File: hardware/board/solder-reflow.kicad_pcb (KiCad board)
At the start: 2 copper layers, 128.3 x 63.5 mm, 55 parts, among them J1 AC_Con, J2 OLED 0.91, J3 PTC_Con, J4 Barrel_Jack_Switch_Pin3Ring, K1 G3MB202PDC12, Q1 BC557, SW1 RotaryEncoder_Switch, U1 TL431LP, U2 OPA2134, U3 OPA2134, U4 L7805, U5 WeMos_D1_mini

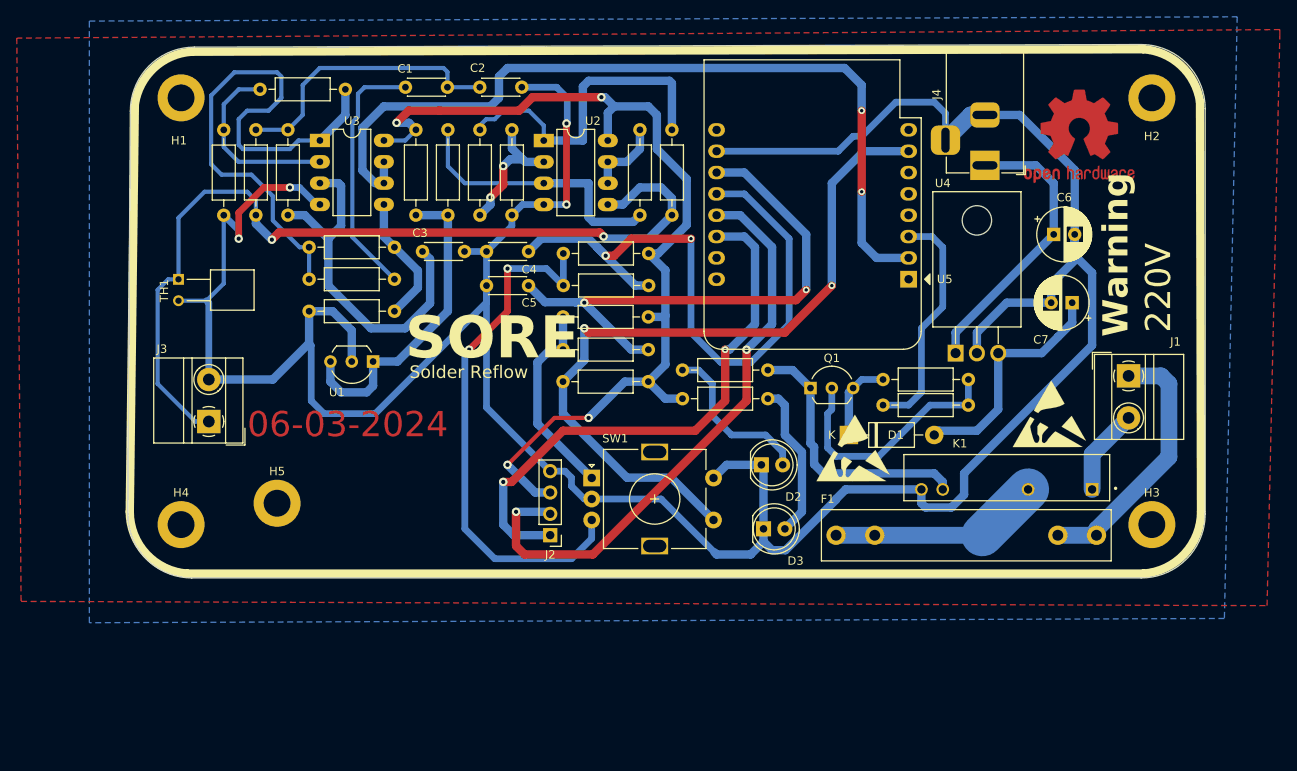
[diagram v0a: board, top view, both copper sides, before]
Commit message: [6-7-1245] finish first layout, need to review
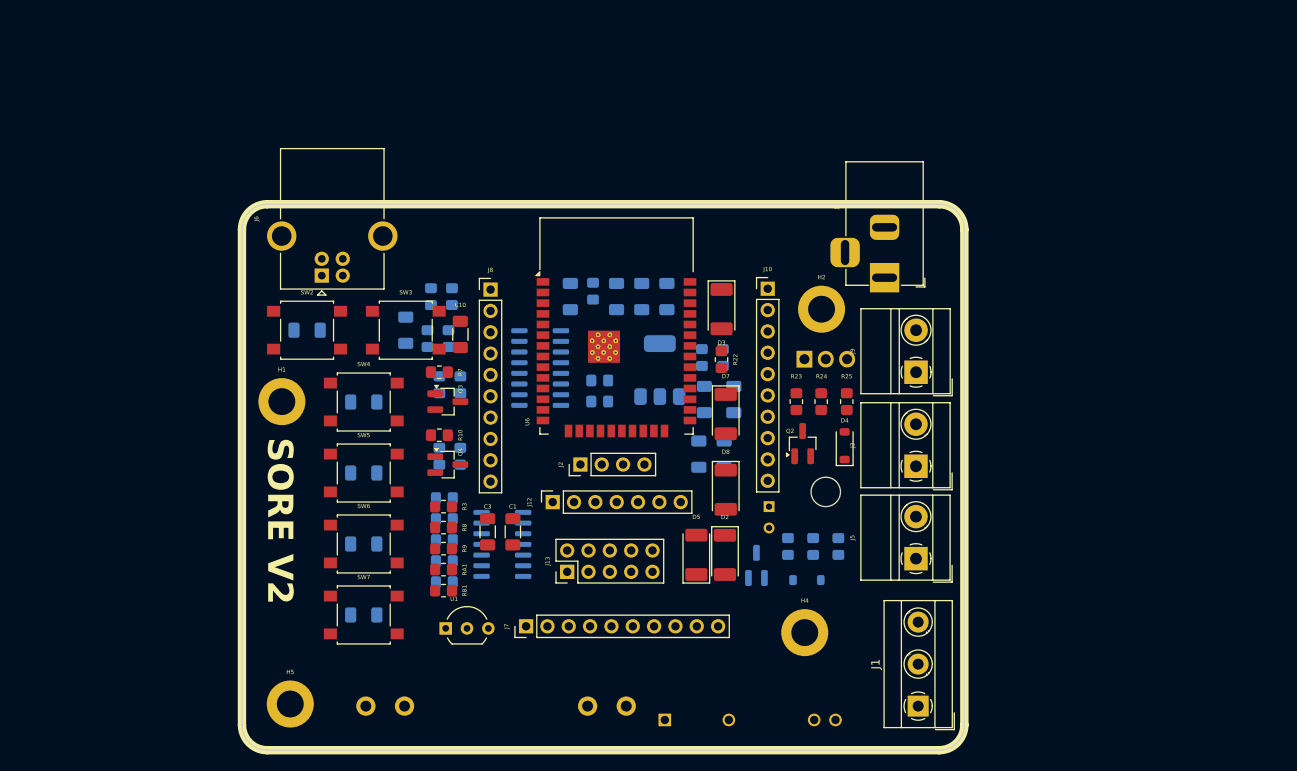
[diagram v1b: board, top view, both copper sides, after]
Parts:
- removed C4, C5: 10nF, Capacitor_THT:C_Disc_D4.3mm_W1.9mm_P5.00mm
- removed H3: MountingHole_Pad, MountingHole:MountingHole_3.2mm_M3_DIN965_Pad
- removed R11, R21: 10k, Resistor_THT:R_Axial_DIN0207_L6.3mm_D2.5mm_P10.16mm_Horizontal
- removed REF**: OSHW-Logo2_14.6x12mm_Copper, Symbol:OSHW-Logo2_14.6x12mm_Copper
- removed REF** (x2): ESD-Logo_8.9x8mm_SilkScreen, Symbol:ESD-Logo_8.9x8mm_SilkScreen
- removed REF**: Gauge_10mm_Type5_SilkScreenTop, Calibration_Scale:Gauge_10mm_Type5_SilkScreenTop
- removed SW1: RotaryEncoder_Switch, Rotary_Encoder:RotaryEncoder_Alps_EC11E-Switch_Vertical_H20mm
- removed U5: WeMos_D1_mini, Module:WEMOS_D1_mini_light
- added C10: 100nF, Capacitor_SMD:C_1206_3216Metric_Pad1.33x1.80mm_HandSolder, F.Cu at (128.5, 81.5)
- added C11: 100nF, Capacitor_SMD:C_1206_3216Metric_Pad1.33x1.80mm_HandSolder, B.Cu at (141.6, 77.0)
- added C12: 100nF, Capacitor_SMD:C_1206_3216Metric_Pad1.33x1.80mm_HandSolder, B.Cu at (150.1, 77.0)
- added C13: 22uF, Capacitor_SMD:C_1206_3216Metric_Pad1.33x1.80mm_HandSolder, B.Cu at (147.1, 77.0)
- added C14: 100nF, Capacitor_SMD:C_1206_3216Metric_Pad1.33x1.80mm_HandSolder, B.Cu at (110.2, 81.0)
- added C15: 100nF, Capacitor_SMD:C_1206_3216Metric_Pad1.33x1.80mm_HandSolder, B.Cu at (122.0, 81.0)
- added C16: 1uF, Capacitor_SMD:C_1206_3216Metric_Pad1.33x1.80mm_HandSolder, B.Cu at (117.0, 89.5)
- added C17: 1uF, Capacitor_SMD:C_1206_3216Metric_Pad1.33x1.80mm_HandSolder, B.Cu at (117.0, 98.0)
- added C18: 1uF, Capacitor_SMD:C_1206_3216Metric_Pad1.33x1.80mm_HandSolder, B.Cu at (117.0, 106.5)
- added C19: 1uF, Capacitor_SMD:C_1206_3216Metric_Pad1.33x1.80mm_HandSolder, B.Cu at (117.0, 114.9)
- added C8: 22uF, Capacitor_SMD:C_1206_3216Metric_Pad1.33x1.80mm_HandSolder, B.Cu at (159.9, 95.8)
- added C9: 22uF, Capacitor_SMD:C_1206_3216Metric_Pad1.33x1.80mm_HandSolder, B.Cu at (156.9, 95.8)
- added D4: 1N4001, Diode_SMD:D_SOD-123, F.Cu at (174.2, 94.8)
- added D5: SSR2, LED_SMD:LED_2010_5025Metric_Pad1.52x2.65mm_HandSolder, F.Cu at (156.6, 107.7)
- added D7: TXD, LED_SMD:LED_2010_5025Metric_Pad1.52x2.65mm_HandSolder, F.Cu at (160.1, 91.0)
- added D8: RXD, LED_SMD:LED_2010_5025Metric_Pad1.52x2.65mm_HandSolder, F.Cu at (160.1, 100.0)
- added J10: PINOUT, Connector_PinHeader_2.54mm:PinHeader_1x10_P2.54mm_Vertical, F.Cu at (165.1, 76.1)
- added J12: ST7789, Connector_PinSocket_2.54mm:PinSocket_1x07_P2.54mm_Vertical, F.Cu at (139.5, 101.5)
- added J13: JTAG10, Connector_PinHeader_2.54mm:PinHeader_2x05_P2.54mm_Vertical, F.Cu at (141.2, 109.8)
- added J5: SSROUT2, TerminalBlock_MetzConnect:TerminalBlock_MetzConnect_Type011_RT05502HBWC_1x02_P5.00mm_Horizontal, F.Cu at (182.7, 108.2)
- added J6: USB_B, Connector_USB:USB_B_OST_USB-B1HSxx_Horizontal, F.Cu at (112.0, 74.5)
- added J7: PINOUT, Connector_PinHeader_2.54mm:PinHeader_1x10_P2.54mm_Vertical, F.Cu at (136.3, 116.2)
- added J8: PINOUT, Connector_PinHeader_2.54mm:PinHeader_1x10_P2.54mm_Vertical, F.Cu at (132.1, 76.2)
- added J9: 12VIN, TerminalBlock_MetzConnect:TerminalBlock_MetzConnect_Type011_RT05502HBWC_1x02_P5.00mm_Horizontal, F.Cu at (182.8, 86.0)
- added Q2: SS8550, Package_TO_SOT_SMD:SOT-23_Handsoldering, F.Cu at (169.2, 94.5)
- added Q3: SS8050, Package_TO_SOT_SMD:SOT-23_Handsoldering, F.Cu at (127.0, 89.5)
- added Q4: SS8050, Package_TO_SOT_SMD:SOT-23_Handsoldering, F.Cu at (127.0, 97.0)
- added R23: 10k, Resistor_SMD:R_0805_2012Metric_Pad1.20x1.40mm_HandSolder, F.Cu at (168.5, 89.5)
- added R24: 10k, Resistor_SMD:R_0805_2012Metric_Pad1.20x1.40mm_HandSolder, F.Cu at (171.4, 89.5)
- added R25: 1k, Resistor_SMD:R_0805_2012Metric_Pad1.20x1.40mm_HandSolder, F.Cu at (174.5, 89.5)
- added R26: 1k, Resistor_SMD:R_0805_2012Metric_Pad1.20x1.40mm_HandSolder, B.Cu at (157.2, 84.2)
- added R27: 1k, Resistor_SMD:R_0805_2012Metric_Pad1.20x1.40mm_HandSolder, B.Cu at (159.8, 84.2)
- added R28: 1k, Resistor_SMD:R_0805_2012Metric_Pad1.20x1.40mm_HandSolder, B.Cu at (144.3, 76.3)
- added R29: 22k, Resistor_SMD:R_0805_2012Metric_Pad1.20x1.40mm_HandSolder, B.Cu at (128.5, 87.5)
- added R30: 22k, Resistor_SMD:R_0805_2012Metric_Pad1.20x1.40mm_HandSolder, B.Cu at (127.1, 82.0)
- added R31: 22k, Resistor_SMD:R_0805_2012Metric_Pad1.20x1.40mm_HandSolder, B.Cu at (127.5, 77.0)
- added R32: 22k, Resistor_SMD:R_0805_2012Metric_Pad1.20x1.40mm_HandSolder, B.Cu at (128.5, 96.0)
- added RA1: 25k, Resistor_SMD:R_0805_2012Metric_Pad1.20x1.40mm_HandSolder, F.Cu at (126.5, 109.5)
- added RB1: 25k, Resistor_SMD:R_0805_2012Metric_Pad1.20x1.40mm_HandSolder, F.Cu at (126.5, 112.0)
- added SW2: RST, Button_Switch_SMD:SW_SPST_B3S-1000, F.Cu at (110.2, 81.0)
- added SW3: IO0, Button_Switch_SMD:SW_SPST_B3S-1000, F.Cu at (122.0, 81.0)
- added SW4: IO0, Button_Switch_SMD:SW_SPST_B3S-1000, F.Cu at (117.0, 89.5)
- added SW5: IO0, Button_Switch_SMD:SW_SPST_B3S-1000, F.Cu at (117.0, 98.0)
- added SW6: IO0, Button_Switch_SMD:SW_SPST_B3S-1000, F.Cu at (117.0, 106.5)
- added SW7: IO0, Button_Switch_SMD:SW_SPST_B3S-1000, F.Cu at (117.0, 114.9)
- added U6: ESP32-WROOM-32D, RF_Module:ESP32-WROOM-32D, F.Cu at (147.1, 83.5)
- added U7: CH340C, Package_SO:SOIC-16_3.9x9.9mm_P1.27mm, B.Cu at (138.0, 85.5)
- C1: value 68nF -> 1nF; footprint Capacitor_THT:C_Disc_D4.3mm_W1.9mm_P5.00mm -> Capacitor_SMD:C_1206_3216Metric_Pad1.33x1.80mm_HandSolder
- C2: value 390nF -> 1uF; footprint Capacitor_THT:C_Disc_D4.3mm_W1.9mm_P5.00mm -> Capacitor_SMD:C_1206_3216Metric_Pad1.33x1.80mm_HandSolder; moved to B.Cu
- C3: value 180nF -> 1nF; footprint Capacitor_THT:C_Disc_D4.3mm_W1.9mm_P5.00mm -> Capacitor_SMD:C_1206_3216Metric_Pad1.33x1.80mm_HandSolder
- C6, C7: footprint Capacitor_THT:CP_Radial_D6.3mm_P2.50mm -> Capacitor_SMD:C_1206_3216Metric_Pad1.33x1.80mm_HandSolder; moved to B.Cu
- D1: footprint Diode_THT:D_DO-41_SOD81_P10.16mm_Horizontal -> Diode_SMD:D_SOD-123; moved to B.Cu
- D2: value SSR -> SSR1; footprint LED_THT:LED_D5.0mm -> LED_SMD:LED_2010_5025Metric_Pad1.52x2.65mm_HandSolder
- D3: footprint LED_THT:LED_D5.0mm -> LED_SMD:LED_2010_5025Metric_Pad1.52x2.65mm_HandSolder
- F1, K1, TH1, U4: moved to B.Cu
- J1: value AC_Con -> ACCON; footprint TerminalBlock_MetzConnect:TerminalBlock_MetzConnect_Type011_RT05502HBWC_1x02_P5.00mm_Horizontal -> TerminalBlock_MetzConnect:TerminalBlock_MetzConnect_Type055_RT01503HDWU_1x03_P5.00mm_Horizontal
- J4: value Barrel_Jack_Switch_Pin3Ring -> 12V
- Q1: value BC557 -> SS8550; footprint Package_TO_SOT_THT:TO-92_Inline_Wide -> Package_TO_SOT_SMD:SOT-23_Handsoldering; moved to B.Cu
- R1, R14, R15, R16, R17, R18, R19, R2, R20, R4, R5, R6: footprint Resistor_THT:R_Axial_DIN0207_L6.3mm_D2.5mm_P10.16mm_Horizontal -> Resistor_SMD:R_0805_2012Metric_Pad1.20x1.40mm_HandSolder; moved to B.Cu
- R10: value 5.1K -> 10k; footprint Resistor_THT:R_Axial_DIN0207_L6.3mm_D2.5mm_P10.16mm_Horizontal -> Resistor_SMD:R_0805_2012Metric_Pad1.20x1.40mm_HandSolder
- R12: value 3.09k -> 4K7; footprint Resistor_THT:R_Axial_DIN0207_L6.3mm_D2.5mm_P10.16mm_Horizontal -> Resistor_SMD:R_0805_2012Metric_Pad1.20x1.40mm_HandSolder; moved to B.Cu
- R13: value 20k -> 4K7; footprint Resistor_THT:R_Axial_DIN0207_L6.3mm_D2.5mm_P10.16mm_Horizontal -> Resistor_SMD:R_0805_2012Metric_Pad1.20x1.40mm_HandSolder; moved to B.Cu
- R22, R3: footprint Resistor_THT:R_Axial_DIN0207_L6.3mm_D2.5mm_P10.16mm_Horizontal -> Resistor_SMD:R_0805_2012Metric_Pad1.20x1.40mm_HandSolder
- R7: value 1k -> 10k; footprint Resistor_THT:R_Axial_DIN0207_L6.3mm_D2.5mm_P10.16mm_Horizontal -> Resistor_SMD:R_0805_2012Metric_Pad1.20x1.40mm_HandSolder
- R8: value 17.4k -> 16k; footprint Resistor_THT:R_Axial_DIN0207_L6.3mm_D2.5mm_P10.16mm_Horizontal -> Resistor_SMD:R_0805_2012Metric_Pad1.20x1.40mm_HandSolder
- R9: value 107k -> 16k; footprint Resistor_THT:R_Axial_DIN0207_L6.3mm_D2.5mm_P10.16mm_Horizontal -> Resistor_SMD:R_0805_2012Metric_Pad1.20x1.40mm_HandSolder
- U2: value OPA2134 -> TL074; footprint Package_DIP:DIP-8_W7.62mm_LongPads -> Package_SO:SOIC-14_3.9x8.7mm_P1.27mm; moved to B.Cu
- U3: value OPA2134 -> AMS1117-3.3; footprint Package_DIP:DIP-8_W7.62mm_LongPads -> Package_TO_SOT_SMD:SOT-223-3_TabPin2; moved to B.Cu
- moved J3 84.4 mm to (182.7, 97.2)
- moved H4 75.4 mm to (169.5, 117.0)
- moved TH1 75.3 mm to (165.2, 102.0)
- moved R1 54.0 mm to (126.6, 111.0), turned to 180 degrees
- moved C1 53.8 mm to (131.8, 105.0), turned to -90 degrees
- moved R13 53.3 mm to (145.1, 87.0), turned to 180 degrees
- moved R8 52.4 mm to (126.5, 104.5), turned to 180 degrees
- moved R12 50.0 mm to (145.1, 89.5), turned to 180 degrees
- moved U3 48.8 mm to (152.2, 85.8), turned to 90 degrees
- moved U2 48.3 mm to (133.5, 106.5), turned to 180 degrees
- moved H2 46.7 mm to (171.5, 78.5)
- moved J1 46.6 mm to (183.0, 125.8), turned to 90 degrees
- moved C7 45.3 mm to (157.6, 89.2), turned to -90 degrees
- moved R4 45.2 mm to (126.6, 106.0), turned to 180 degrees
- moved R3 44.1 mm to (126.5, 102.0), turned to 180 degrees
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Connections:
- net /pt100_out renamed /PT100Voltage
- net Net-(U4-IN) renamed +12V
- C1 pad 1: Net-(C1-Pad1) -> Net-(U2D-+)
- C2 pad 1: Net-(C1-Pad2) -> +3.3V
- C3 pad 1: Net-(U3A-+) -> Net-(U2C-+)
- F1 pad 1: Net-(K1-L2) -> AC
- F1 pad 2: AC -> Net-(K1-L2)
- J1 pad 2: Net-(J1-Pin_2) -> unconnected-(J1-Pin_2-Pad2)
- J2 pad 1: /OLED_SCL -> /I2C_SDA
- J2 pad 2: /OLED_SDA -> /I2C_SCL
- K1 pad 1: Net-(J1-Pin_2) -> Net-(J1-Pin_3)
- Q1 pad 1: Net-(K1-+) -> Net-(Q1-B)
- Q1 pad 2: Net-(Q1-B) -> Net-(D1-K)
- Q1 pad 3: Net-(D1-K) -> Net-(K1-+)
- R1 pad 1: +5V -> +2V5
- R1 pad 2: +2V5 -> +5V
- R10 pad 1: Net-(R10-Pad1) -> Net-(Q4-B)
- R10 pad 2: Net-(U3B-+) -> /RTS
- R12 pad 1: GND -> /I2C_SDA
- R12 pad 2: Net-(U3A--) -> +3.3V
- R13 pad 1: Net-(U3A--) -> /I2C_SCL
- R13 pad 2: Net-(R10-Pad1) -> +3.3V
- R15 pad 1: /SSR_in -> /SSRIN1
- R16 pad 1: Net-(R16-Pad1) -> +3.3V
- R16 pad 2: +5V -> Net-(R16-Pad2)
- R17 pad 1: Net-(R17-Pad1) -> +3.3V
- R17 pad 2: +5V -> Net-(R17-Pad2)
- R19 pad 1: /ENC_SW -> +3.3V
- R19 pad 2: +5V -> Net-(R19-Pad2)
- R20 pad 1: Net-(R16-Pad1) -> +3.3V
- R20 pad 2: /ENC_A -> Net-(R20-Pad2)
- R7 pad 1: Net-(R10-Pad1) -> Net-(Q3-B)
- R7 pad 2: Net-(C1-Pad1) -> /DTR
- R9 pad 1: Net-(U3A-+) -> Net-(U2C-+)
- U2 pad 4: GND -> +5V
- U2 pad 8: +5V -> Net-(U2D-+)
- U3 pad 1: Net-(R10-Pad1) -> GND
- U3 pad 2: Net-(U3A--) -> +3.3V
- U3 pad 3: Net-(U3A-+) -> +5V
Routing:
- net GND: track 364.4 -> 0.00 mm, vias 4 -> 0
- net +5V: track 144.5 -> 0.00 mm, vias 4 -> 0
- net /PT100Voltage: track 106.3 -> 0.00 mm, vias 2 -> 0
- net /Sallen-Key_out: track 100.6 -> 0.00 mm, vias 2 -> 0
- net /ENC_SW: track 89.3 -> 0.00 mm, vias 2 -> 0
- net /ENC_A: track 76.9 -> 0.00 mm, vias 2 -> 0
- net /OLED_SDA: track 71.7 -> 0.00 mm, vias 2 -> 0
- net Net-(R10-Pad1): track 68.5 -> 0.00 mm
- net /OLED_SCL: track 66.8 -> 0.00 mm, vias 2 -> 0
- net /ENC_B: track 65.8 -> 0.00 mm, vias 2 -> 0
- net Net-(R16-Pad1): track 64.2 -> 0.00 mm, vias 2 -> 0
- net Net-(U3A-+): track 43.1 -> 0.00 mm
- net Net-(R3-Pad2): track 39.0 -> 0.00 mm
- net +2V5: track 37.8 -> 0.00 mm
- net +12V: track 34.1 -> 0.00 mm
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- removed copper zone on F.Cu, net +5V
- removed copper zone on B.Cu, net GND
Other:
- board size 128.3 x 63.5 mm -> 86 x 65 mm
- board text added: "SORE V2"
- board text removed: "06-03-2024"
- board text removed: "220V"
- board text removed: "SORE"
- board text removed: "Solder Reflow"
- board text removed: "V1 Custom PTC Heater Controller for SMD Solder-Reflow"
- board text removed: "Warning"
